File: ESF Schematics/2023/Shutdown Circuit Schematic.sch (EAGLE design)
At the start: 80 parts, among them J1 CONNECTOR-1_LCAX2-14F-E, J2 CONNECTOR-1_LCAX2-14F-E, J3 CONNECTOR-1_LCAX2-14F-E, J4 CONNECTOR-1_LCAX2-14F-E, Q1 MOSFET_N-CHANNEL, Q2 MOSFET_N-CHANNEL, U1 LOGICGATE_INVERTER, U2 LOGICGATE_INVERTER

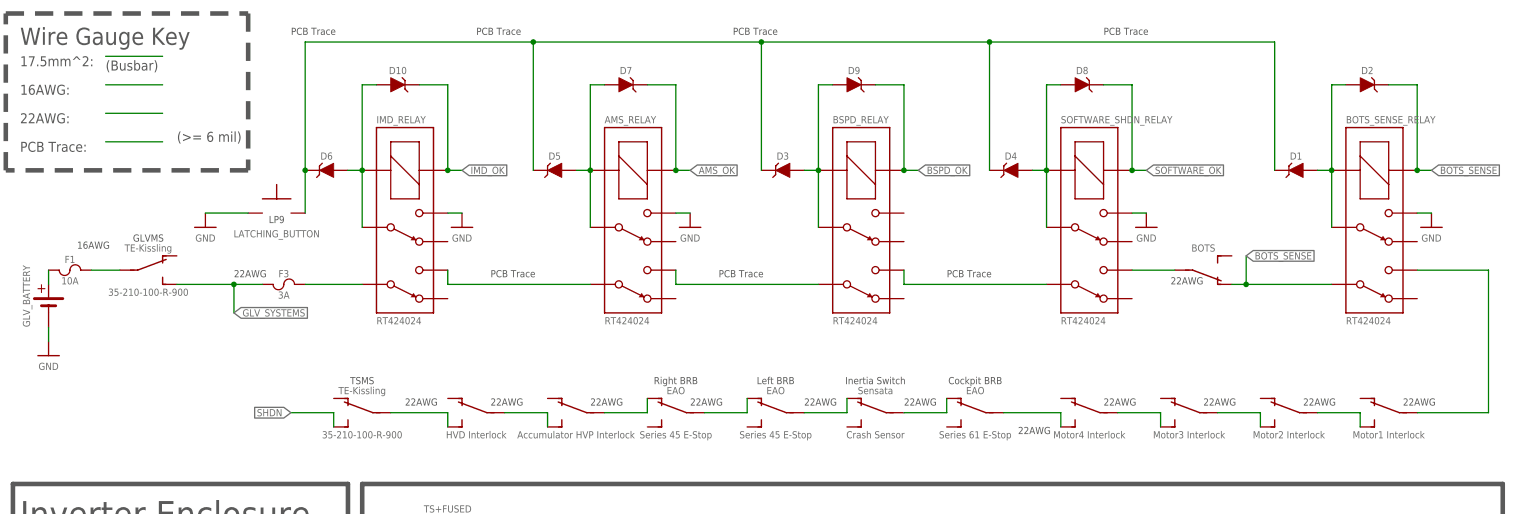
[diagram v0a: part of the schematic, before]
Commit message: TS big changes
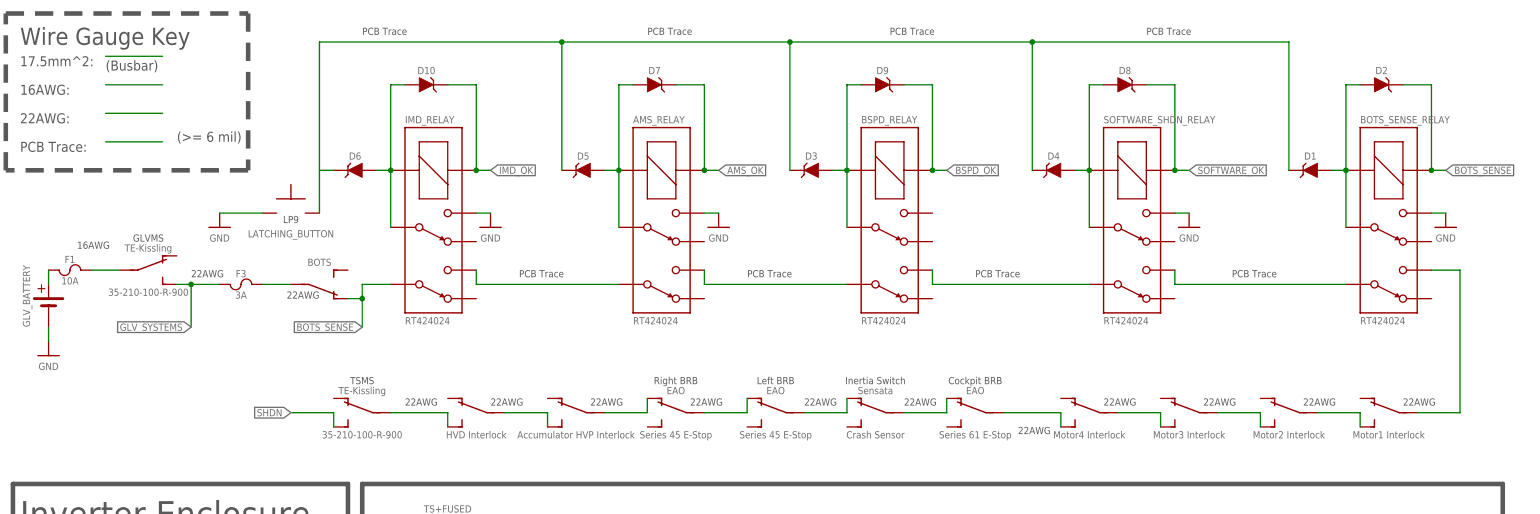
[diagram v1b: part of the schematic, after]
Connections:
- net BOTS_SENSE: now also IMD_RELAY.6; no longer BOTS_SENSE_RELAY.6
- net N$15: now also BOTS_SENSE_RELAY.6; no longer S2.P
- net N$22: now also S2.P; no longer IMD_RELAY.6
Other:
- moved on the sheet: AMS_RELAY, BOTS_SENSE_RELAY, BSPD_RELAY, D1, D10, D2, D3, D4, D5, D6, D7, D8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
